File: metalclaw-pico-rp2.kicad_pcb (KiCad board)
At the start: 4 copper layers, 21 x 51 mm, 123 parts, among them J1 USB4105-GF-A, J2 FTSH-105-01-L-DV-K, SW1 PTS810SJM250SMTR LFS, SW2 PTS810SJM250SMTR LFS, U1 XC6220B331MR-G, U2 RP2354B, U3 APS6404L-3SQR-SN, Y1 ABM8-272-T3

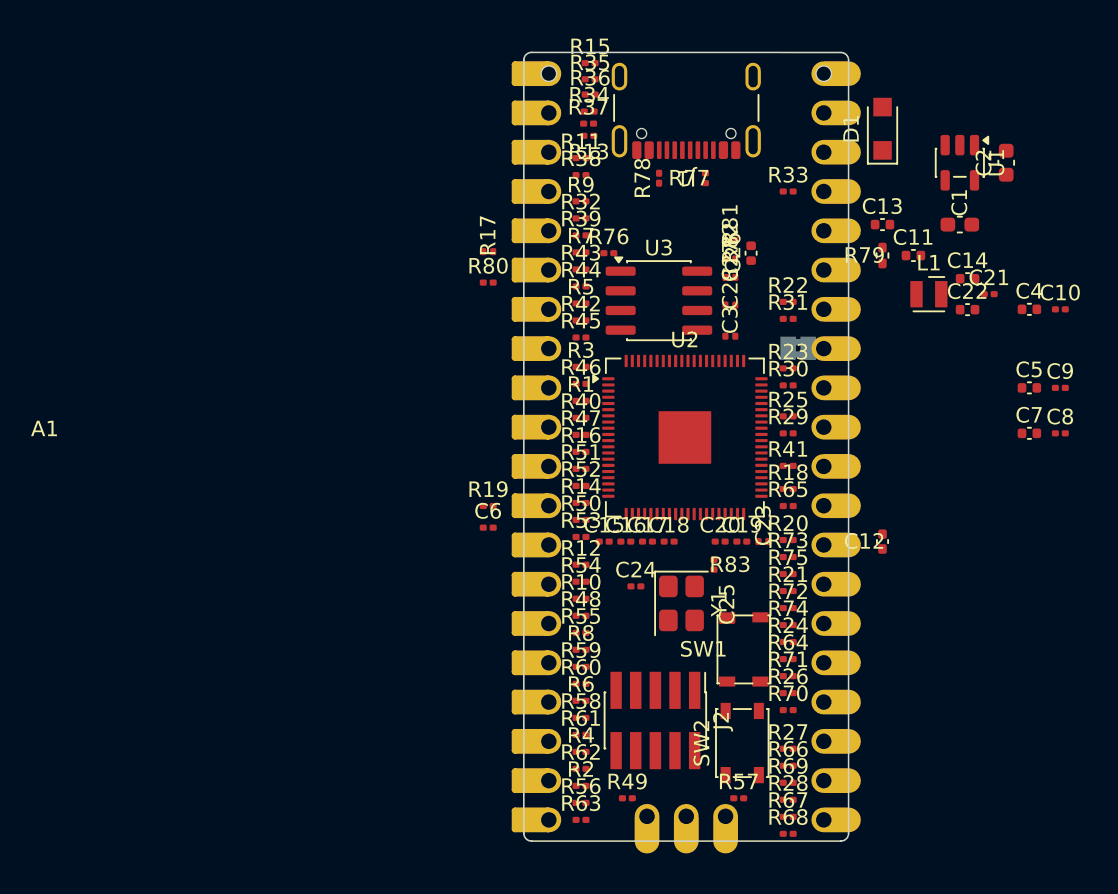
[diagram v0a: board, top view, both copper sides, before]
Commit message: More initial rough placement
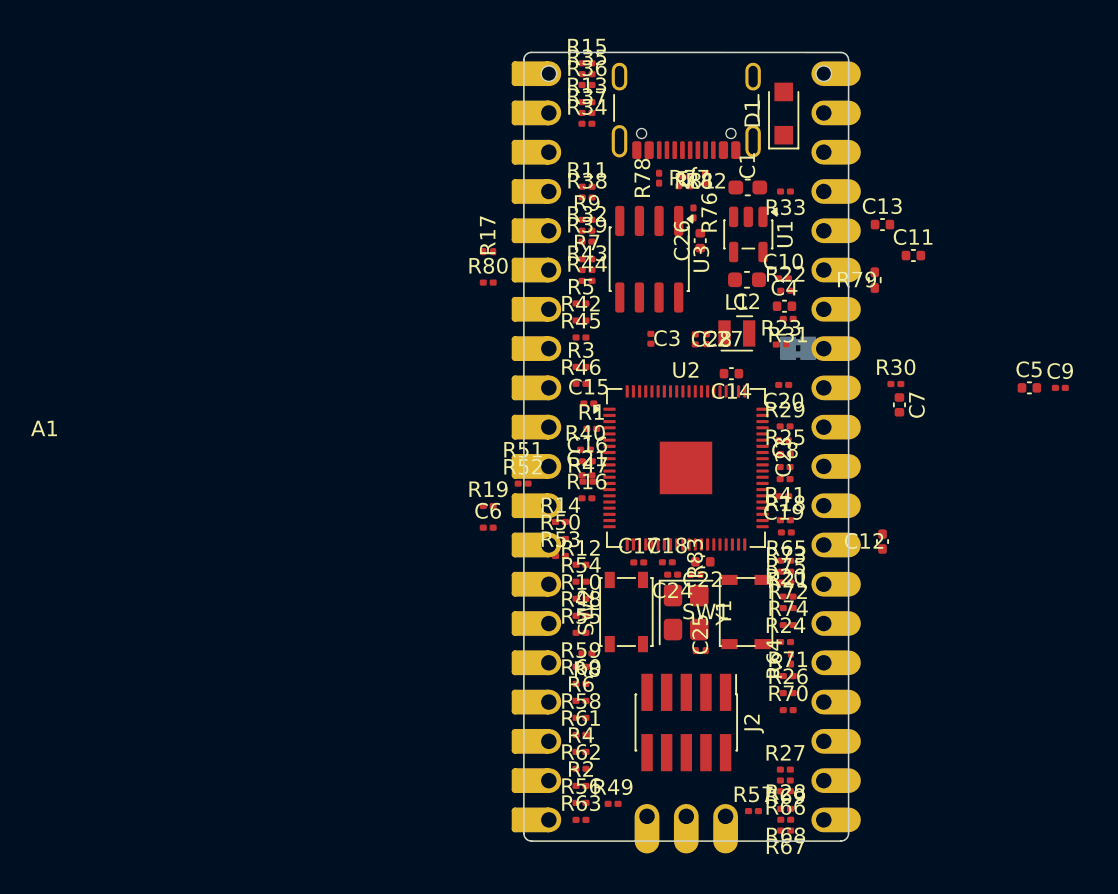
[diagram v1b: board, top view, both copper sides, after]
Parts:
- moved C21 28.5 mm to (157.4, 100.7)
- moved C22 23.6 mm to (164.9, 106.3), turned to 180 degrees
- moved C2 18.4 mm to (167.7, 88.1), turned to 180 degrees
- moved C10 18.0 mm to (170.1, 88.0)
- moved C8 17.9 mm to (170.2, 100.2)
- moved C14 16.5 mm to (166.7, 94.1), turned to 180 degrees
- moved C4 15.8 mm to (170.2, 89.8)
- moved U1 14.4 mm to (167.8, 85.1)
- moved C1 13.9 mm to (167.8, 82.1)
- moved L1 12.7 mm to (167.1, 91.5)
- moved SW2 11.3 mm to (159.9, 109.6)
- moved C20 10.9 mm to (170.1, 94.9), turned to 180 degrees
- moved C15 8.99 mm to (157.5, 96.1)
- moved C7 8.60 mm to (177.6, 96.2), turned to -90 degrees
- moved R30 6.97 mm to (177.4, 94.8)
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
